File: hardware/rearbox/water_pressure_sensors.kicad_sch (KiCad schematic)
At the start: 8 parts

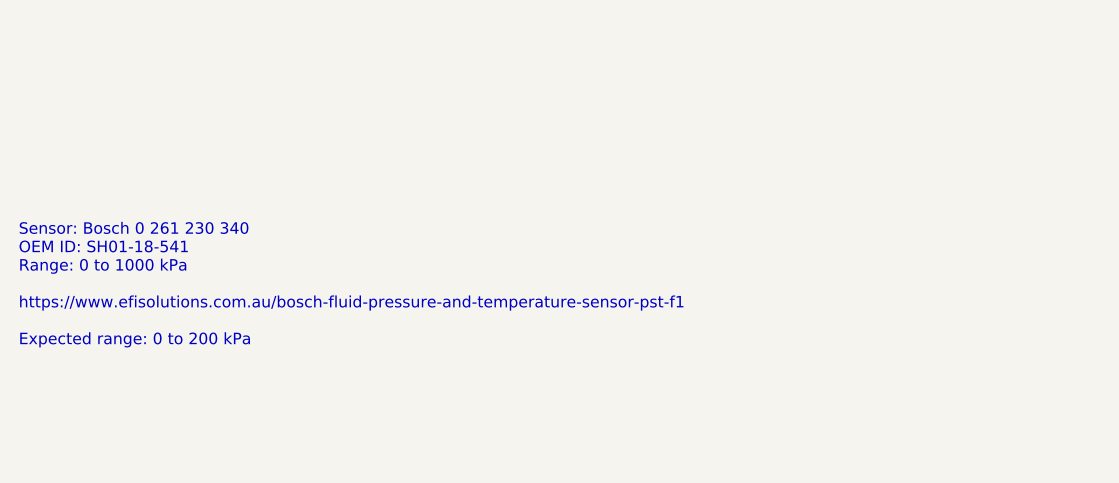
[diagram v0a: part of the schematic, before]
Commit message: Changed power section
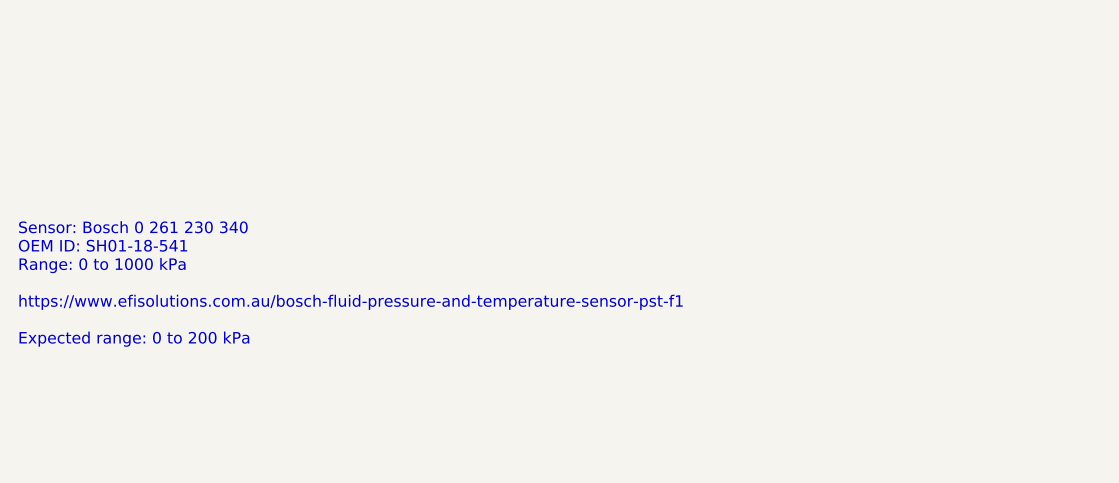
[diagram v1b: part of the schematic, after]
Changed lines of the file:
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@@
 (kicad_sch
-	(version 20231120)
+	(version 20250114)
 	(generator "eeschema")
-	(generator_version "8.0")
+	(generator_version "9.0")
 	(paper "A4")
 	(title_block
@@
 		(comment 1 "Reviewer:")
 	)
+	(text "0.5 V"
+		(exclude_from_sim no)
+		(at 165.1 77.47 0)
+		(effects
+			(font
+				(size 1.27 1.27)
+			)
+			(justify right bottom)
+		)
+	)
+	(text "0.5 V"
+		(exclude_from_sim no)
+		(at 165.1 130.81 0)
+		(effects
+			(font
+				(size 1.27 1.27)
+			)
+			(justify right bottom)
+		)
+	)
+	(text "0.5 to 1.3 V"
+		(exclude_from_sim no)
+		(at 171.45 55.88 0)
+		(effects
+			(font
+				(size 1.27 1.27)
+			)
+			(justify right bottom)
+		)
+	)
+	(text "G = 2\nR_{F} = 4k7\nR_{G} = 4k7"
+		(exclude_from_sim no)
+		(at 207.01 128.27 0)
+		(effects
+			(font
+				(size 1.27 1.27)
+			)
+			(justify left bottom)
+		)
+	)
+	(text "G = 2\nR_{F} = 4k7\nR_{G} = 4k7"
+		(exclude_from_sim no)
+		(at 207.01 74.93 0)
+		(effects
+			(font
+				(size 1.27 1.27)
+			)
+			(justify left bottom)
+		)
+	)
+	(text "0.5 to 1.3 V"
+		(exclude_from_sim no)
+		(at 171.45 109.22 0)
+		(effects
+			(font
+				(size 1.27 1.27)
+			)
+			(justify right bottom)
+		)
+	)
+	(text_box "Sensor: Bosch 0 261 230 340\nOEM ID: SH01-18-541\nRange: 0 to 1000 kPa\n\nhttps://www.efisolutions.com.au/bosch-fluid-pressure-and-temperature-sensor-pst-f1\n\nExpected range: 0 to 200 kPa"
+		(exclude_from_sim no)
+		(at 21.59 115.57 0)
+		(size 88.9 15.24)
+		(margins 0.9524 0.9524 0.9524 0.9524)
+		(stroke
+			(width -0.0001)
+			(type default)
+		)
+		(fill
+			(type none)
+		)
+		(effects
+			(font
+				(size 1.27 1.27)
+			)
+			(justify left top)
+		)
+	)
 	(junction
 		(at 185.42 129.54)
@@
 			"AABMgOIOAAAATIDiDgAAAEyA4g4AAABMgOIOAAAATIDiDgAAAEyA4g4AAABMgOIOAAAATIDiDgAA"
 			"AEyA4g4AAABMgOIOAAAATIDiDgAAAEyA4g4AAABMgOIOAAAATIDiDgAAAEzgX51T7NJvUuP9AAAA"
-			"AElFTkSuQmCC"
-		)
-	)
-	(text_box "Sensor: Bosch 0 261 230 340\nOEM ID: SH01-18-541\nRange: 0 to 1000 kPa\n\nhttps://www.efisolutions.com.au/bosch-fluid-pressure-and-temperature-sensor-pst-f1\n\nExpected range: 0 to 200 kPa"
-		(exclude_from_sim no)
-		(at 21.59 115.57 0)
-		(size 88.9 15.24)
-		(stroke
-			(width -0.0001)
-			(type default)
-		)
-		(fill
-			(type none)
-		)
-		(effects
-			(font
-				(size 1.27 1.27)
-			)
-			(justify left top)
-		)
-	)
-	(text "0.5 V"
-		(exclude_from_sim no)
-		(at 165.1 77.47 0)
-		(effects
-			(font
-				(size 1.27 1.27)
-			)
-			(justify right bottom)
-		)
-	)
-	(text "0.5 V"
-		(exclude_from_sim no)
-		(at 165.1 130.81 0)
-		(effects
-			(font
-				(size 1.27 1.27)
-			)
-			(justify right bottom)
-		)
-	)
-	(text "0.5 to 1.3 V"
-		(exclude_from_sim no)
-		(at 171.45 55.88 0)
-		(effects
-			(font
-				(size 1.27 1.27)
-			)
-			(justify right bottom)
-		)
-	)
-	(text "G = 2\nR_{F} = 4k7\nR_{G} = 4k7"
-		(exclude_from_sim no)
-		(at 207.01 128.27 0)
-		(effects
-			(font
-				(size 1.27 1.27)
-			)
-			(justify left bottom)
-		)
-	)
-	(text "G = 2\nR_{F} = 4k7\nR_{G} = 4k7"
-		(exclude_from_sim no)
-		(at 207.01 74.93 0)
-		(effects
-			(font
-				(size 1.27 1.27)
-			)
-			(justify left bottom)
-		)
-	)
-	(text "0.5 to 1.3 V"
-		(exclude_from_sim no)
-		(at 171.45 109.22 0)
-		(effects
-			(font
-				(size 1.27 1.27)
-			)
-			(justify right bottom)
+			"AElFTkSuQmCCAE0AcQAzAEIAVgBGAFUAUgBSAEYAaQBaAG8AbABEAEMARAAvAFEAdwBxAHkAagAx"
+			"AHMAYgBmAGMAcwBSADUAWABVAHAAegAzADEATAB2AHUAVwBQAGcAQgBOAHgARgAxADMATABKAFgA"
+			"aQBoAEUASAA4AFcAQwBUAGoAUQBhAHkARABHAGIAUwBKAFIAZgBLAGsAUAArAGQAYgBEAG0ASwBn"
+			"AC8ATwBvADUAdwBtAFgAaABLAFIARQBnAFEATQBuAFgAWgBZADkAagBBADAAeAB6AGYAQwArAGUA"
+			"VABjAFkAVgBtAEEAcQBIAFAAMQBhAHMALwByADkAUwBOADIAZgBPADQAaABIAGoAMABXAHgAWABT"
+			"AGUAdQA2AHcAZwBOAHUALwBjAHEAVgA4AGsANwBLAGIAOQArAFEARQBOAGQASQB5ADcAaABxADAA"
+			"VABiAGEALwBzAG4AdgBvAHkAcQBtAEsAbwBpAGkASwBvAHQAUQB0AGEALwAvADIAMgAyADkALwA5"
+			"ADkAMQAzAGkASABqAGMAQwBjAGUAUABHAEQARgBDAGgASwBtAEUAVgB4AEcAeAB0AHIAWgAyADMA"
+			"cgB4ADUAaQB4AFkAdABLAGkAOAB0AHkAOAB6AE0ASABEAHAAMAA2AEwAQgBoAHcAOQBDAEwAeQBU"
+			"ADEAUwA1AHgAaABCACsATwByAEwATAA3AC8ANAA2AHMAdQB0AFcANwBlAG0AcAA2AFkAZABkAHQA"
+			"aABoAHcANABjAFAAVAAwAGwASgBDAFkAVgBDAHYARgBRAG4AQwB6ADUAVwBnAFUAUwAwAGQAdQAz"
+			"AGEAagB6AC8AKwBlAE0ATwBHAEQAVQBsAEoAUwBUADEANwA5AHoAcgB0AHQATgBOAHkAYwAzAFAA"
+			"UgBzAFoAVwBMAFIAawBUAEUAegBaAHMAMwBmAC8AVABoADMARABWAHIAMQBoAEIAQwBYAGwANwBl"
+			"AHEAYQBlAGUAMgByADEANwBkADQAegAxAG8ARABmAEcAcQA2ACsAKwB1AG4AbgB6AFoAZwBCAEkA"
+			"VAAwADgAZgBQADMANAA4AEoASgB6AFAAdQBuAEQAaAB3AG8AOAArACsAaQBqAE8AagBZAE8ASQBv"
+			"AFYAQQBvAE4AVABVADEASwB5AHUAcgBiADkAKwArAFIAeAB3ACsAVQBPAHgARAAwAE0AcQBNAEkA"
+			"dQA2AHcAaQBkAFIALwArAC8AYgB0AHoAegB6AHoARABHAHYAMwBhADYANgA1AHAAbgBQAG4AegBo"
+			"AGgAcgBXADYAOABQAEUAYQAxAGEAdABXAHIAOQArAHYAWABTAFUASgBJADMAaABqADkANAAyAEcA"
+			"RwBIAGQAZQ=="
 		)
 	)
@@
 		(shape input)
 		(at 180.34 107.95 180)
-		(fields_autoplaced yes)
 		(effects
 			(font
@@
 		(shape output)
 		(at 224.79 107.95 0)
-		(fields_autoplaced yes)
 		(effects
 			(font
@@
 		(shape input)
 		(at 180.34 54.61 180)
-		(fields_autoplaced yes)
 		(effects
 			(font
@@
 		(shape output)
 		(at 224.79 54.61 0)
-		(fields_autoplaced yes)
 		(effects
 			(font
@@
 		(at 199.39 50.8)
 		(size 24.13 13.97)
+		(exclude_from_sim no)
+		(in_bom yes)
+		(on_board yes)
+		(dnp no)
 		(stroke
 			(width 0.1524)
@@
 		(at 199.39 104.14)
 		(size 24.13 13.97)
+		(exclude_from_sim no)
+		(in_bom yes)
+		(on_board yes)
+		(dnp no)
 		(stroke
 			(width 0.1524)
